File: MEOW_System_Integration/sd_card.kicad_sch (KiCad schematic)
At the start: 10 parts, among them IC1 LM1117MPX-3.3_NOPB, J5 Conn_01x06_Pin, J6 MEM2090-00-145-00-A, J7 Conn_01x04_Pin

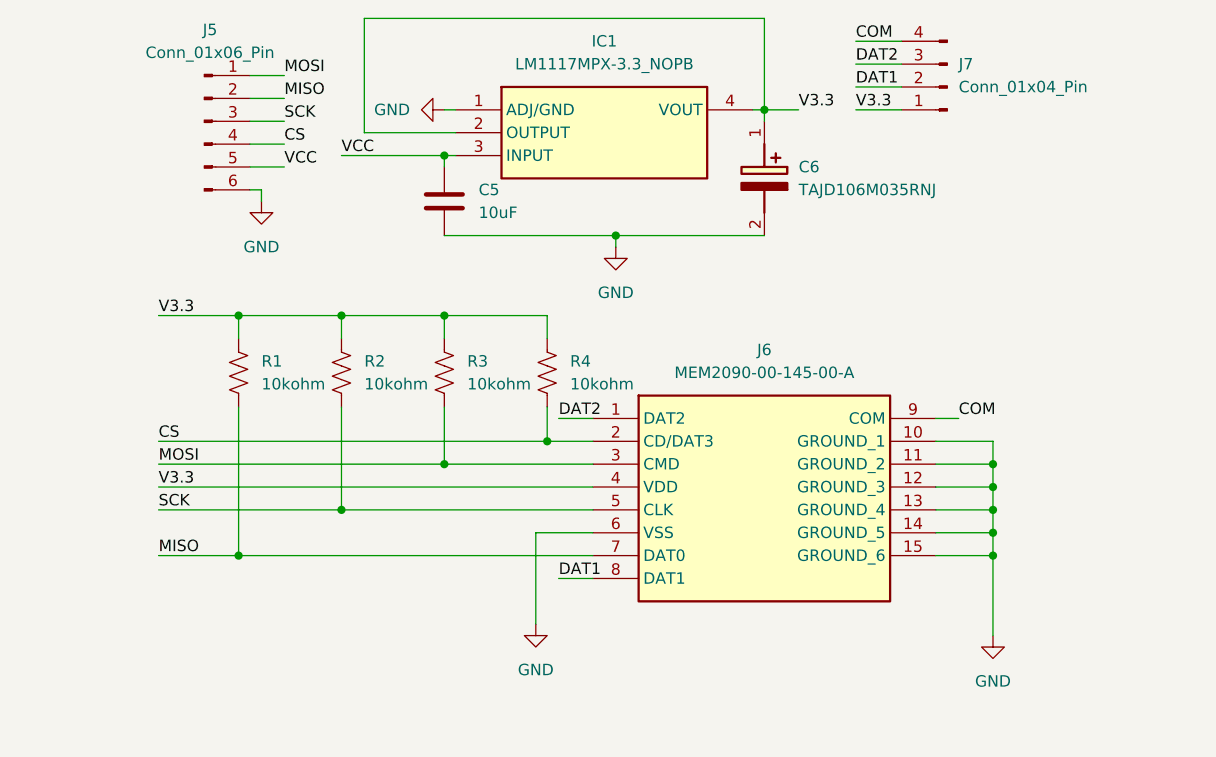
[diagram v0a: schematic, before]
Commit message: current status PCB ordered
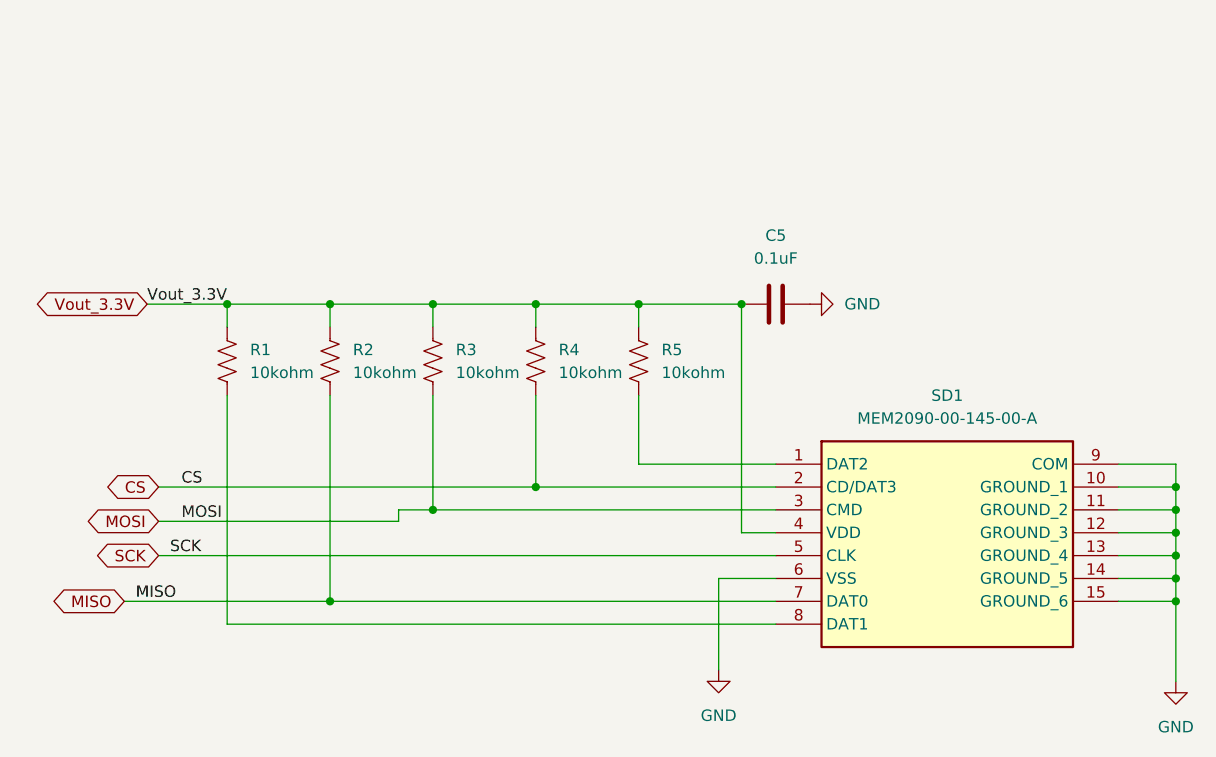
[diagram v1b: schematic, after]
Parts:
- removed C6: TAJD106M035RNJ, CAPPM7344X310N, symbol SamacSys_Parts:TAJD106M035RNJ
- removed IC1: LM1117MPX-3.3_NOPB, SOT230P700X180-4N, symbol SamacSys_Parts:LM1117MPX-3.3_NOPB
- removed J5: Conn_01x06_Pin, Connector_PinHeader_2.54mm:PinHeader_1x06_P2.54mm_Vertical, symbol Connector:Conn_01x06_Pin
- removed J7: Conn_01x04_Pin, Connector_PinHeader_2.54mm:PinHeader_1x04_P2.54mm_Vertical, symbol Connector:Conn_01x04_Pin
- added R5: 10kohm, Resistor_SMD:R_0603_1608Metric_Pad0.98x0.95mm_HandSolder, symbol Device:R_US
- C5: value 10uF -> 0.1uF; footprint Capacitor_SMD:C_1206_3216Metric_Pad1.33x1.80mm_HandSolder -> Capacitor_SMD:C_0603_1608Metric
- SD1: renamed from J6; footprint MEM20900014500A -> footprints:MEM20900014500A
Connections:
- net COM is gone; now on net GND: SD1.9 (COM)
- net VCC is gone; now on net GND: C5.2
- net GND: no longer C5.1
- net MISO: now also R2.2; no longer R1.2
- net SCK: no longer R2.2
- net DAT1: no longer names the net of SD1.8 (DAT1)
- net DAT1: now also R1.2
- net DAT2: no longer names the net of SD1.1 (DAT2)
- net DAT2: now also R5.2
- net V3.3 renamed Vout_3.3V
- net Vout_3.3V: now also C5.1, R5.1
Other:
- moved on the sheet: R1, R2, R3, R4, SD1
